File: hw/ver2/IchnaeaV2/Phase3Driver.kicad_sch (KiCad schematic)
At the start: 21 parts, among them Q10 MCAC80N10Y, Q11 MCAC80N10Y, Q12 MCAC80N10Y, Q13 MCAC80N10Y, U4 HIP2210

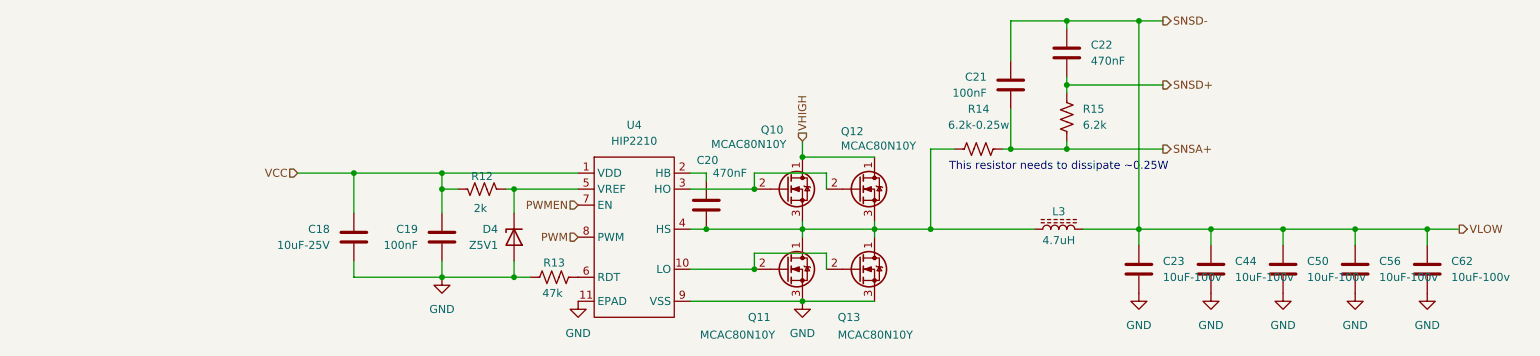
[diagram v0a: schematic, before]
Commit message: Sync work to main PC
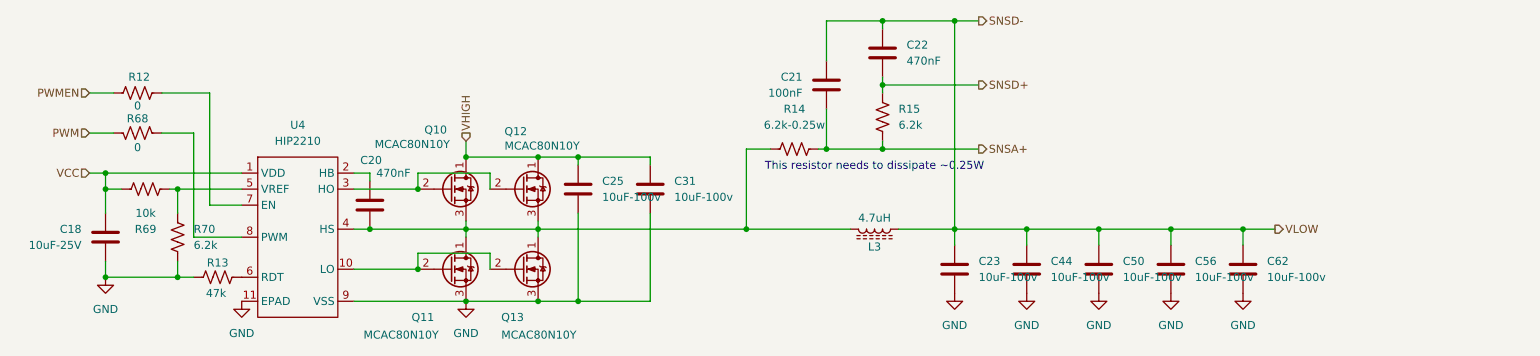
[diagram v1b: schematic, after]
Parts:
- removed C19: 100nF, Capacitor_SMD:C_0603_1608Metric, symbol Device:C
- removed D4: Z5V1, Diode_SMD:D_SOD-123, symbol Device:D_Zener
- added C25, C31: 10uF-100v, Capacitor_SMD:C_1210_3225Metric_Pad1.33x2.70mm_HandSolder, symbol Device:C
- added R68: 0, Resistor_SMD:R_0603_1608Metric, symbol Device:R_US
- added R69: 10k, Resistor_SMD:R_0603_1608Metric, symbol Device:R_US
- added R70: 6.2k, Resistor_SMD:R_0603_1608Metric, symbol Device:R_US
- R12: value 2k -> 0; LCSC (none) -> C21189
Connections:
- net GND: now also C25.2, C31.2, R70.2
- net PWM: now also R68.2; no longer U4.8 (PWM)
- net PWMEN: now also R12.2; no longer U4.7 (EN)
- net SNSD-: now also L3.1; no longer L3.2
- net VCC: now also R69.1; no longer R12.2
- net VHIGH: now also C25.1, C31.1
- net at C20.2, Q10.3 (S), Q11.1 (D)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: now also L3.2; no longer L3.1
- net at R12.1: now also U4.7 (EN); no longer U4.5 (VREF)
- new net: R69.2, R70.1, U4.5 (VREF)
- new net: R68.1, U4.8 (PWM)
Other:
- moved on the sheet: C18, C20, C21, C22, C23, C44, C50, C56, C62, L3, Q10, Q11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
